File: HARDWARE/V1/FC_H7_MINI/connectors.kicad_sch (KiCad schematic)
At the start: 33 parts, among them J2 SM08B-SRSS-TB, J3 SM06B-SRSS-TB, M1 TestPoint_Small, M2 TestPoint_Small, M3 TestPoint_Small, M4 TestPoint_Small

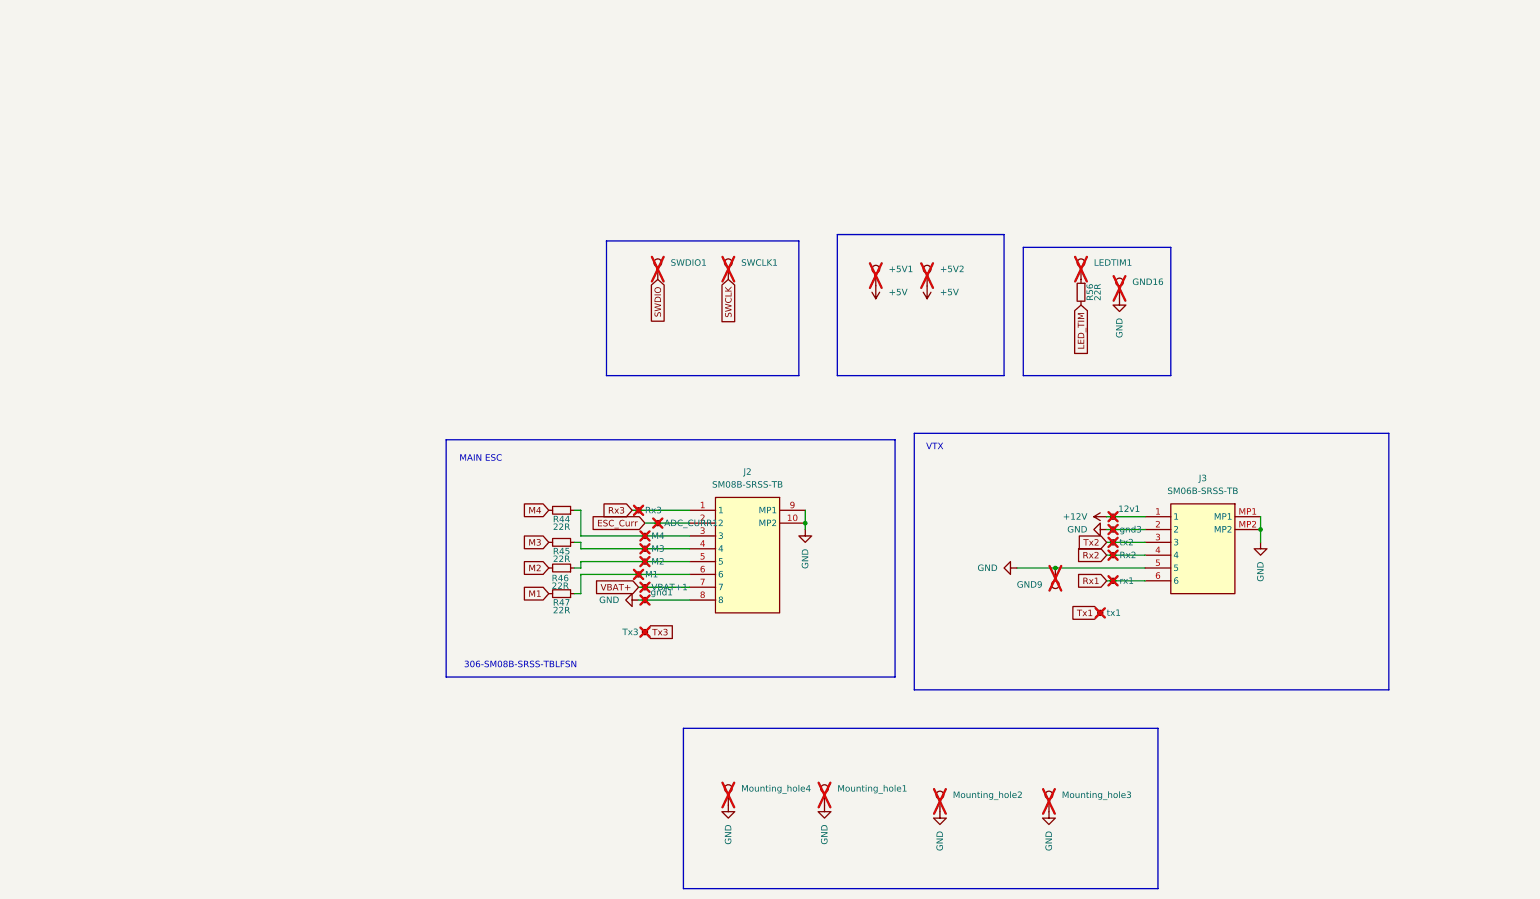
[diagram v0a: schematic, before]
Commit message: up
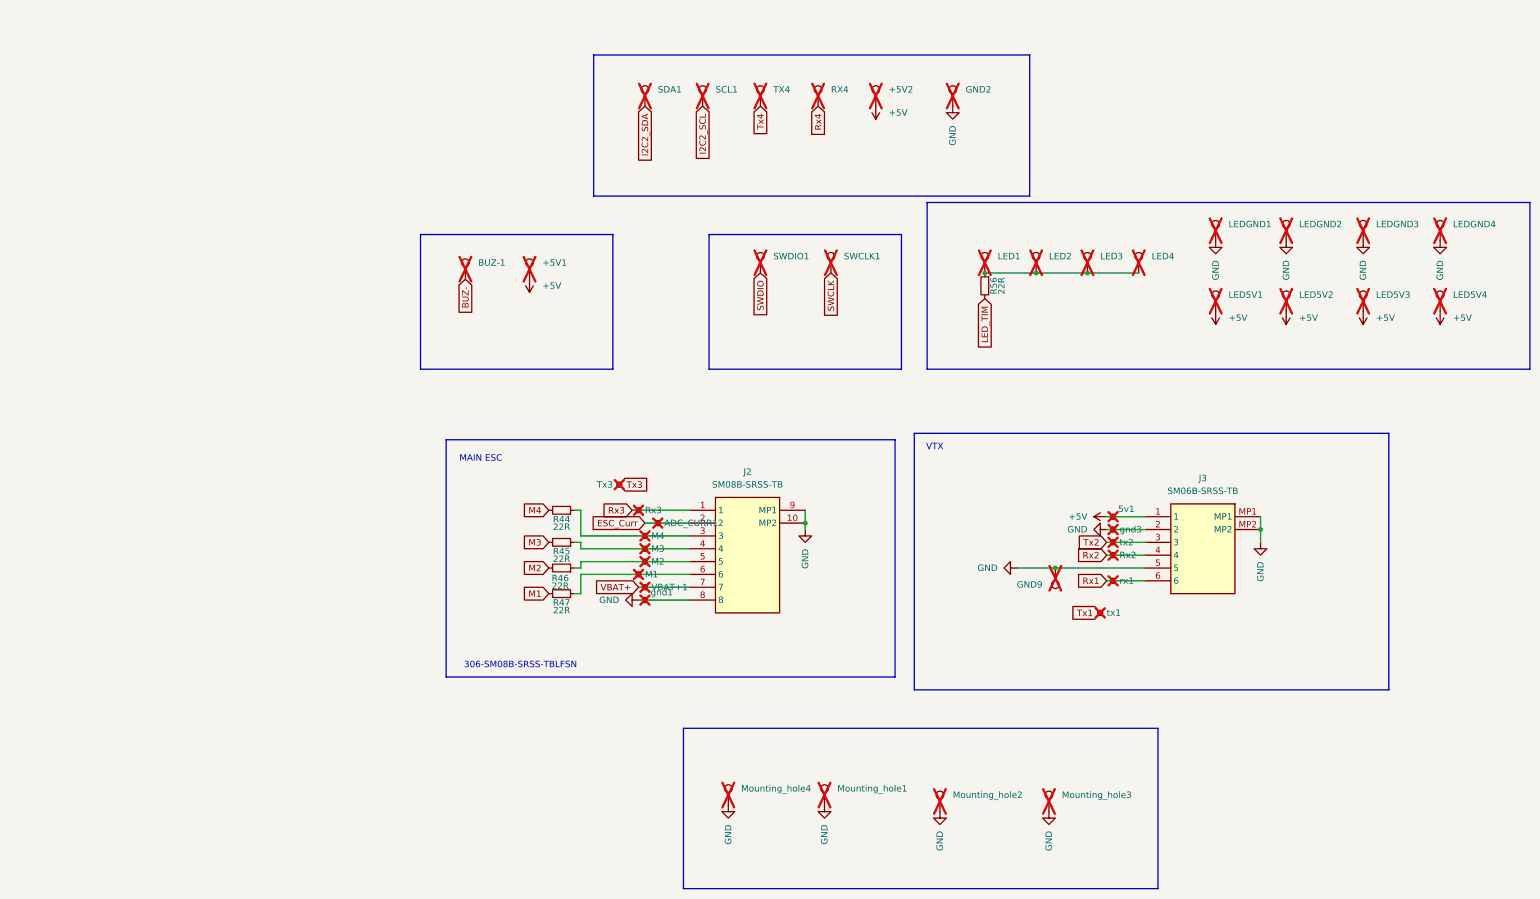
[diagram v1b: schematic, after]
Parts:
- removed GND16, LEDTIM1: TestPoint, fc_h7:1.5mmx1.5mm, symbol Connector:TestPoint
- added +5V1, BUZ-1, RX4, SCL1, SDA1, TX4: TestPoint, samacsys2:PAD_1.5mmx1.5mm, symbol Connector:TestPoint
- added LED1, LED2, LED3, LED4, LED5V1, LED5V2, LED5V3, LED5V4, LEDGND1, LEDGND2, LEDGND3, LEDGND4: TestPoint, samacsys2:1mm_circle, symbol Connector:TestPoint
- +5V2: footprint fc_h7:1.5mmx1.5mm -> samacsys2:PAD_1.5mmx1.5mm
- 5v1: renamed from 12v1; footprint fc_h7:pads_1.5x1.5 -> samacsys2:PAD_1.5mmx1.5mm_hole
- ADC_CURR1, GND9, M1, M2, M3, M4, Rx2, Rx3, Tx3, VBAT+1, gnd1, gnd3, rx1, tx1, tx2: footprint fc_h7:pads_1.5x1.5 -> samacsys2:PAD_1.5mmx1.5mm_hole
- GND2: renamed from +5V1; footprint fc_h7:1.5mmx1.5mm -> samacsys2:PAD_1.5mmx1.5mm
- SWCLK1, SWDIO1: footprint fc_h7:test_point_1MMx1MM -> samacsys2:1mm_circle
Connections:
- net +12V is gone; now on net +5V: 5v1.1, J3.1
- net +5V: now also +5V1.1, LED5V1.1, LED5V2.1, LED5V3.1, LED5V4.1; no longer GND2.1
- net GND: now also GND2.1, LEDGND1.1, LEDGND2.1, LEDGND3.1, LEDGND4.1
- net at R56.1: now also LED1.1, LED2.1, LED3.1, LED4.1
- new net BUZ-: BUZ-1.1
- new net I2C2_SCL: SCL1.1
- new net I2C2_SDA: SDA1.1
- new net Rx4: RX4.1
- new net Tx4: TX4.1
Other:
- moved on the sheet: +5V2, GND2, R56, SWCLK1, SWDIO1, Tx3

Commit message: up
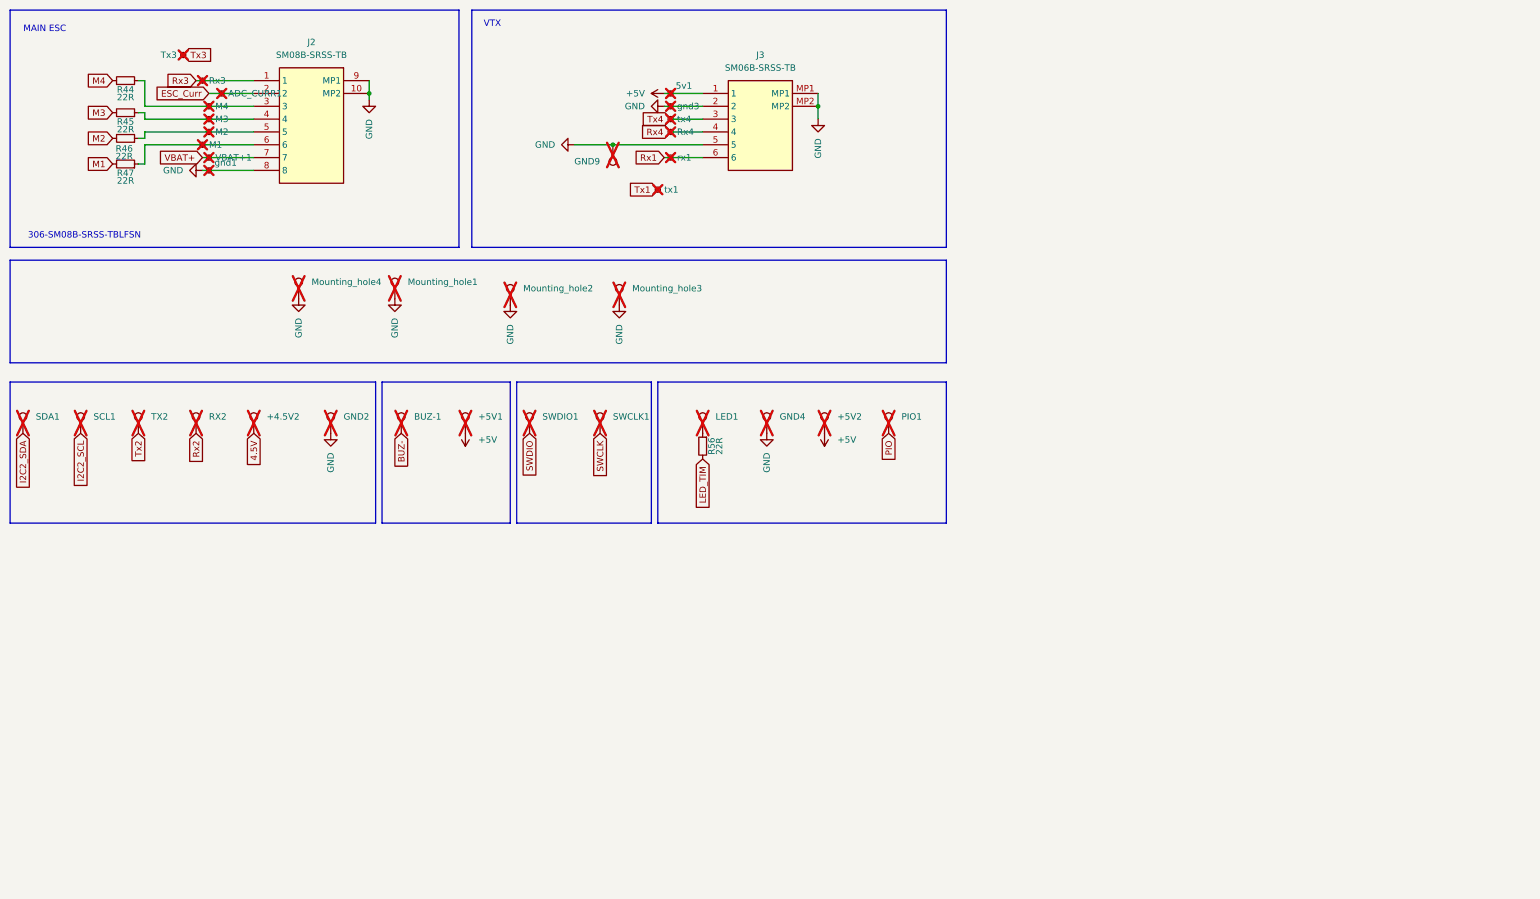
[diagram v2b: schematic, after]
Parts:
- removed LED2, LED3, LED4, LED5V1, LED5V2, LED5V3, LED5V4, LEDGND1, LEDGND2, LEDGND3, LEDGND4: TestPoint, samacsys2:1mm_circle, symbol Connector:TestPoint
- added +5V2, GND4, PIO1: TestPoint, samacsys2:PAD_1.5mmx1.5mm, symbol Connector:TestPoint
- LED1: footprint samacsys2:1mm_circle -> samacsys2:PAD_1.5mmx1.5mm
- renumbered +5V2 to +4.5V2, RX4 to RX2, Rx2 to Rx4, TX4 to TX2, tx2 to tx4
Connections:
- net +5V: now also +5V2.1; no longer +4.5V2.1
- net GND: now also GND4.1
- net Rx2: now also RX2.1; no longer J3.4, Rx4.1
- net Rx4: now also J3.4, Rx4.1; no longer RX2.1
- net Tx2: now also TX2.1; no longer J3.3, tx4.1
- net Tx4: now also J3.3, tx4.1; no longer TX2.1
- new net 4.5V: +4.5V2.1
- new net PIO: PIO1.1
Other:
- moved on the sheet: +4.5V2, +5V1, 5v1, ADC_CURR1, BUZ-1, GND2, GND9, J2, J3, M1, M2, M3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
